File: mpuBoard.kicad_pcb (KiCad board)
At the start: 2 copper layers, 67 parts, among them J1 USB_B_Micro, J2 USB_B, Q1 bss138, Q2 bss138, Q3 bss138, SW1 SW_Push, SW2 SW_Push, U1 AT91SAM9N12, U2 ACT8865, U3 as4c128m8d2-25bin, U4 S34ML08G201TFI, Y1 16MHz, Y2 32.768kHz

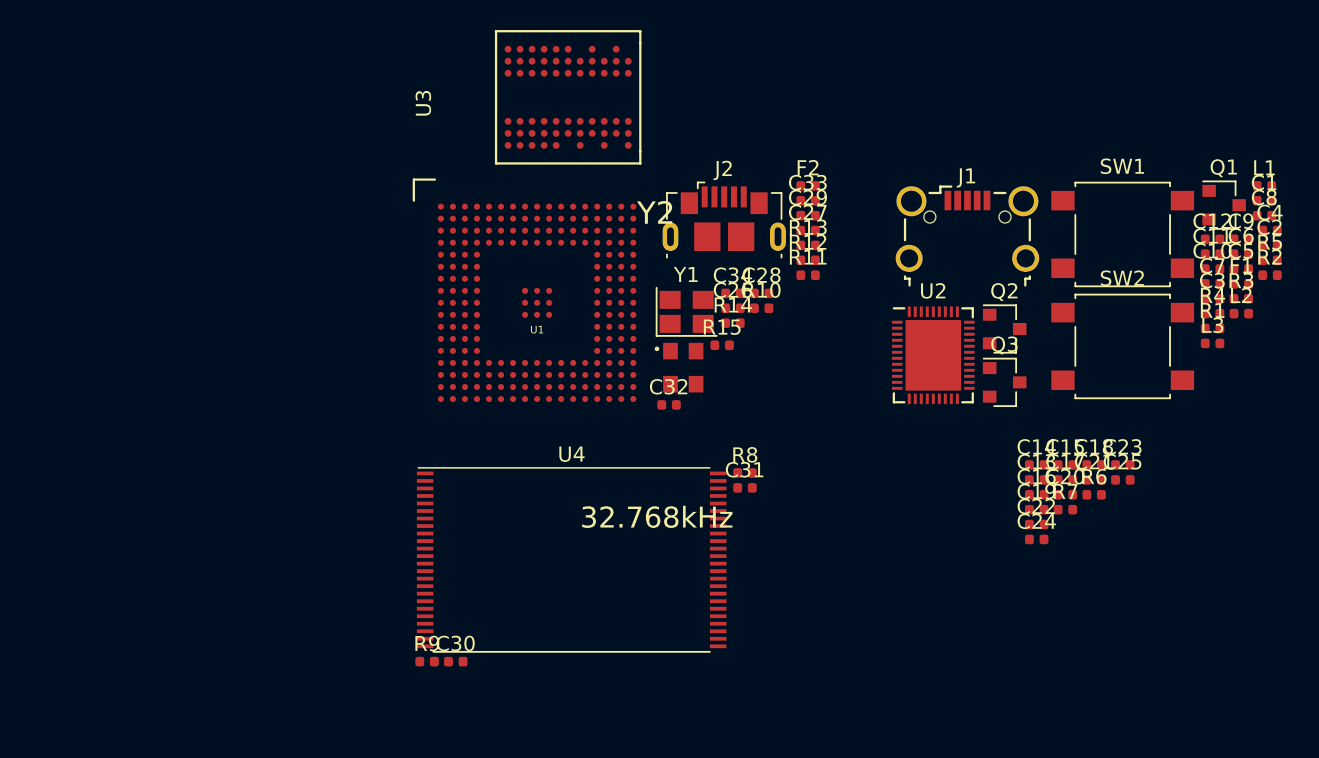
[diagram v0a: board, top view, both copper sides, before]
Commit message: Ordered boards
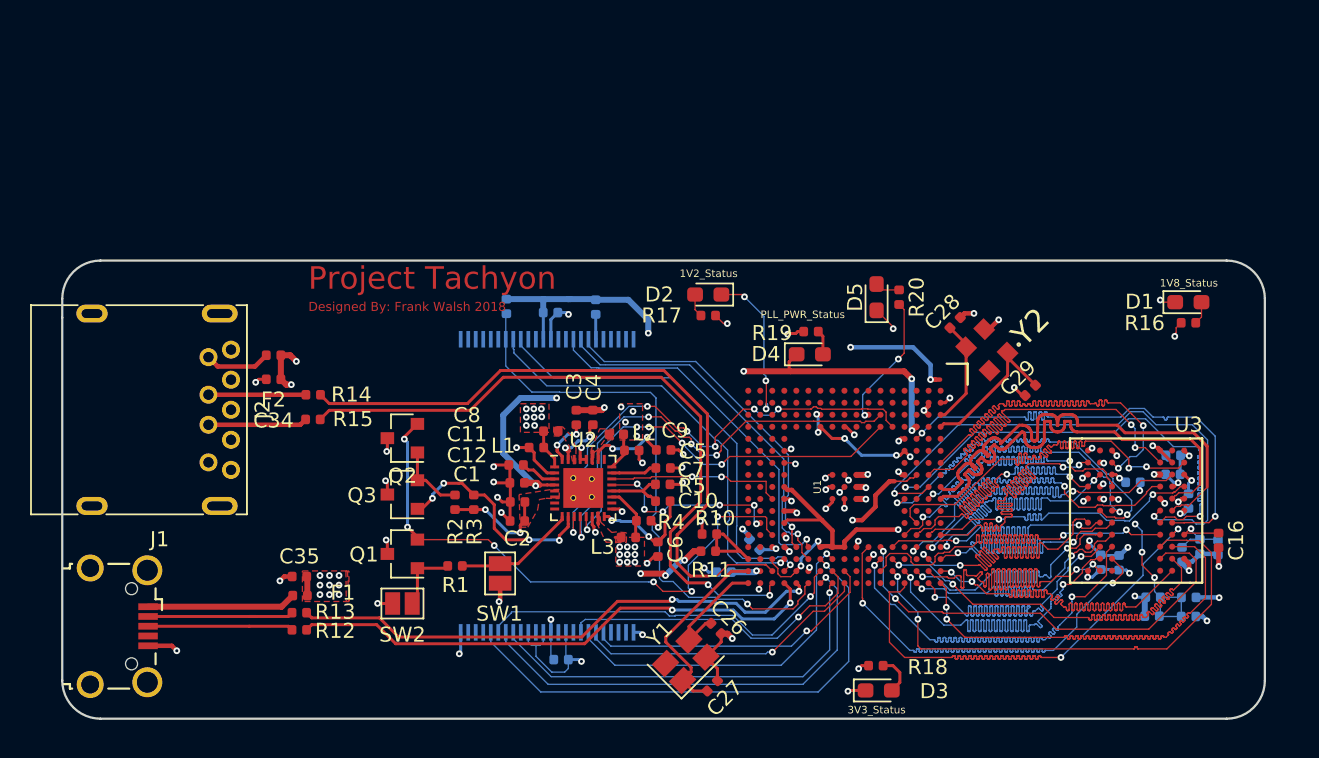
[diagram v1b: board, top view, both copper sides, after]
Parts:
- removed C22: 100n, Capacitor_SMD:C_0402_1005Metric
- added C35: C_Small, Capacitor_SMD:C_0402_1005Metric, F.Cu at (85.6, 102.3)
- added D1: LED, LED_SMD:LED_0603_1608Metric_Pad1.05x0.95mm_HandSolder, F.Cu at (144.8, 84.0)
- added D2: LED, LED_SMD:LED_0603_1608Metric_Pad1.05x0.95mm_HandSolder, F.Cu at (112.8, 83.5)
- added D3: LED, LED_SMD:LED_0603_1608Metric_Pad1.05x0.95mm_HandSolder, F.Cu at (124.2, 109.9)
- added D4: LED, LED_SMD:LED_0603_1608Metric_Pad1.05x0.95mm_HandSolder, F.Cu at (119.6, 87.5)
- added D5: LED, LED_SMD:LED_0603_1608Metric_Pad1.05x0.95mm_HandSolder, F.Cu at (124.0, 83.7)
- added R16: R, Resistor_SMD:R_0402_1005Metric, F.Cu at (144.8, 85.4)
- added R17: R, Resistor_SMD:R_0402_1005Metric, F.Cu at (112.8, 84.9)
- added R18: R, Resistor_SMD:R_0402_1005Metric, F.Cu at (124.0, 108.2)
- added R19: R, Resistor_SMD:R_0402_1005Metric, F.Cu at (119.7, 86.0)
- added R20: 10k, Resistor_SMD:R_0402_1005Metric, F.Cu at (125.5, 83.7)
- C13, C14, C15, C17, C18, C19, C20, C21, C23, C24, C25, C30, C31, C32, C33, R6, R7, R8, R9, U4: moved to B.Cu
- J2: value USB_B -> USB_A; footprint Connector_USB:USB_Micro-B_GCT_USB3076-30-A -> Connector_USB:USB3_A_Molex_48393-001
- SW1, SW2: footprint Button_Switch_SMD:SW_SPST_B3S-1000 -> Jumper:SolderJumper-2_P1.3mm_Open_Pad1.0x1.5mm
- U2: footprint Package_DFN_QFN:QFN-42-1EP_5x6mm_P0.4mm_EP3.7x4.7mm -> Package_DFN_QFN:QFN-32-1EP_4x4mm_P0.4mm_EP2.65x2.65mm
- moved F1 66.0 mm to (85.7, 103.6), turned to 180 degrees
- moved J1 62.3 mm to (73.7, 105.6), turned to 270 degrees
- moved Q1 59.4 mm to (92.5, 100.8), turned to 180 degrees
- moved R2 56.3 mm to (96.0, 97.4), turned to 90 degrees
- moved C1 53.6 mm to (100.1, 97.3), turned to 180 degrees
- moved C2 53.3 mm to (100.1, 98.6), turned to 180 degrees
- moved R3 52.8 mm to (97.2, 97.4), turned to 90 degrees
- moved R1 52.8 mm to (96.0, 101.6), turned to 180 degrees
- moved SW2 50.9 mm to (92.5, 104.1)
- moved C8 50.8 mm to (101.4, 93.7), turned to 180 degrees
- moved L1 50.2 mm to (102.4, 92.6), turned to 180 degrees
- moved C12 49.0 mm to (100.1, 96.1), turned to 180 degrees
- moved C11 48.4 mm to (100.0, 94.9), turned to 180 degrees
- moved SW1 47.2 mm to (99.0, 102.1), turned to 90 degrees
- moved C4 46.7 mm to (105.2, 91.7), turned to 270 degrees
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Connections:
- net Net-(R12-Pad2) renamed /mpu/microD+
- net Net-(R13-Pad2) renamed /mpu/microD-
- net Net-(R14-Pad1) renamed /mpu/fullD-
- net Net-(R15-Pad1) renamed /mpu/fullD+
- C30 pad 1: Net-(C30-Pad1) -> +3V3
- U1 pad A13: /mpu/d6 -> /memory/d6
- U1 pad A14: /mpu/d1 -> /memory/d1
- U1 pad B13: /mpu/d5 -> /memory/d5
- U1 pad B14: /mpu/d0 -> /memory/d0
- U1 pad C12: /mpu/d7 -> /memory/d7
- U1 pad C13: /mpu/d4 -> /memory/d4
- U1 pad C14: /mpu/d2 -> /memory/d2
- U1 pad D13: /mpu/d3 -> /memory/d3
- U1 pad E4: Net-(U1-PadE4) -> /mpu/actGPIO0
- U1 pad F3: Net-(U1-PadF3) -> /mpu/actGPIO1
- U1 pad F4: Net-(U1-PadF4) -> /mpu/actGPIO2
- U2 pad 33: (no net) -> GND
- U4 pad 12: Net-(C30-Pad1) -> +3V3
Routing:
- net GND: track 0.00 -> 84.9 mm, vias 0 -> 71
- net +3V3: track 0.00 -> 69.5 mm, vias 0 -> 26
- net out5: track 0.00 -> 65.5 mm, vias 0 -> 7
- net /mpu/fullD+: track 0.00 -> 46.8 mm, vias 0 -> 2
- net /mpu/fullD-: track 0.00 -> 46.1 mm
- net /memory/a12: track 0.00 -> 39.7 mm, vias 0 -> 2
- net /mpu/flashCTL4: track 0.00 -> 38.6 mm, vias 0 -> 1
- net /mpu/mpu_shutdown: track 0.00 -> 38.6 mm, vias 0 -> 6
- net /memory/ramsel1: track 0.00 -> 36.3 mm, vias 0 -> 2
- net /memory/a7: track 0.00 -> 36.1 mm, vias 0 -> 2
- net /mpu/microD+: track 0.00 -> 36.1 mm, vias 0 -> 2
- net /mpu/microD-: track 0.00 -> 36.0 mm, vias 0 -> 2
- net /memory/d2: track 0.00 -> 34.3 mm, vias 0 -> 2
- net /mpu/flashData0: track 0.00 -> 34.3 mm, vias 0 -> 1
- net /memory/ramsel2: track 0.00 -> 34.1 mm, vias 0 -> 2
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- added copper zone on F.Cu, net +1V2
- added copper zone on VCC, net +1V2
- added copper zone on F.Cu, net +1V8
- added copper zone on VCC, net +1V8
- added copper zone on F.Cu, net +3V3
- added copper zone on VCC, net +3V3
- added copper zone on F.Cu, net +5V
- added copper zone on VCC, net +5V
- added copper zone on F.Cu, net /power/sw1
- added copper zone on F.Cu, net /power/sw2
- added copper zone on F.Cu, net /power/sw3
- added copper zone on GND, net GND
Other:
- board outline added: 80 x 30.5 mm
- copper layers 2 -> 4
- board text added: "1V2_Status"
- board text added: "1V8_Status"
- board text added: "3V3_Status"
- board text added: "Designed By: Frank Walsh 2018"
- board text added: "PLL_PWR_Status"
- board text added: "Project Tachyon"
